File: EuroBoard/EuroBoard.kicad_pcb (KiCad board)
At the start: 2 copper layers, 100 x 100 mm, 21 parts, among them J1 SPI, SW1 RESET, SW2 BOOT, U1 AMS1117-3.3, U2 STM32G030CxT, Y1 NX2520 16MHz

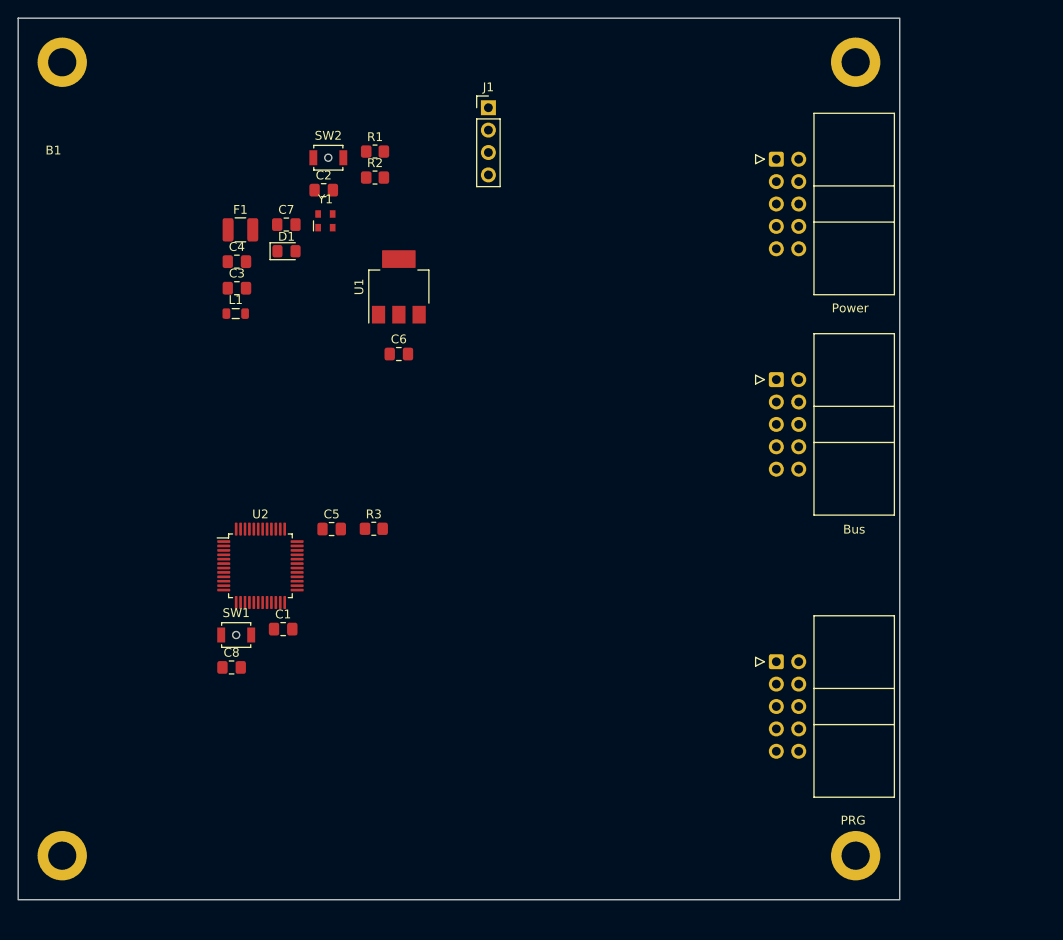
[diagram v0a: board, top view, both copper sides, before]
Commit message: Started doing PCB
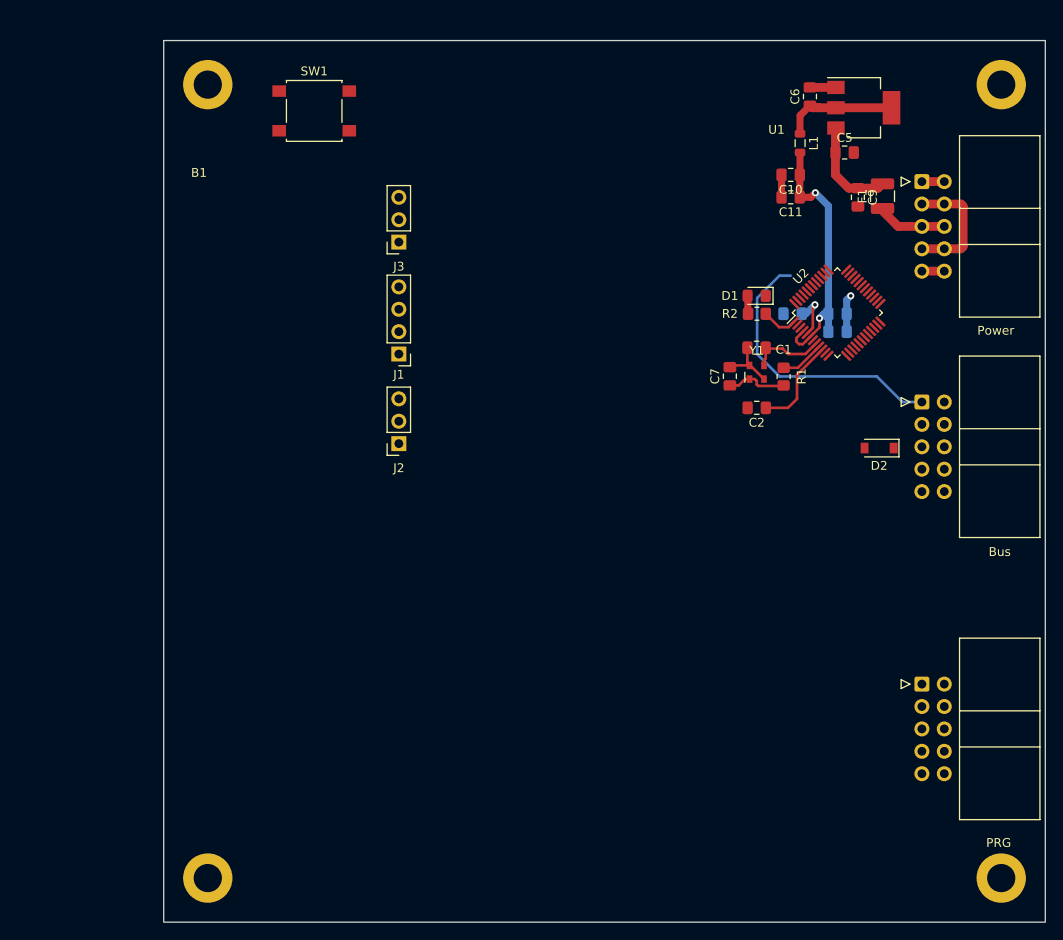
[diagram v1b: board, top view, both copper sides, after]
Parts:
- removed R3: R, Resistor_SMD:R_0805_2012Metric_Pad1.20x1.40mm_HandSolder
- removed SW2: BOOT, Button_Switch_SMD:SW_SPST_B3U-1000P-B
- added C10: 100n, Capacitor_SMD:C_0805_2012Metric_Pad1.18x1.45mm_HandSolder, F.Cu at (146.1, 48.3)
- added C11: 10u, Capacitor_SMD:C_0805_2012Metric_Pad1.18x1.45mm_HandSolder, F.Cu at (146.1, 50.8)
- added C9: 10u, Capacitor_SMD:C_0805_2012Metric_Pad1.18x1.45mm_HandSolder, F.Cu at (153.7, 50.8)
- added D2: 1n4148, Diode_SMD:D_SOD-123, F.Cu at (156.1, 79.2)
- added J2: I2C, Connector_PinSocket_2.54mm:PinSocket_1x03_P2.54mm_Vertical, F.Cu at (101.6, 78.7)
- added J3: UART, Connector_PinSocket_2.54mm:PinSocket_1x03_P2.54mm_Vertical, F.Cu at (101.6, 55.9)
- C3, C8: moved to B.Cu
- C4: value 4.7u -> 10u; moved to B.Cu
- SW1: footprint Button_Switch_SMD:SW_SPST_B3U-1000P-B -> Button_Switch_SMD:SW_SPST_B3S-1000
- moved C8 75.2 mm to (146.3, 64.0), turned to 180 degrees
- moved F1 72.9 mm to (156.5, 50.7), turned to 90 degrees
- moved C5 72.2 mm to (152.2, 45.7)
- moved U2 71.5 mm to (151.3, 63.9), turned to 45 degrees
- moved C4 68.6 mm to (151.4, 66.0)
- moved C3 68.2 mm to (151.4, 64.0)
- moved L1 66.9 mm to (147.1, 44.7), turned to -90 degrees
- moved C1 62.5 mm to (142.2, 67.9), turned to 180 degrees
- moved SW1 60.1 mm to (92.0, 41.0)
- moved U1 56.5 mm to (154.3, 40.6), turned to 0 degrees
- moved C6 55.0 mm to (148.2, 39.4), turned to 90 degrees
- moved C2 55.0 mm to (142.2, 74.7), turned to 180 degrees
- moved D1 53.6 mm to (142.2, 62.0), turned to 180 degrees
- moved C7 53.2 mm to (139.1, 71.1), turned to 90 degrees
- moved R1 52.9 mm to (145.2, 71.1), turned to 90 degrees
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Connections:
- net Net-(R2-Pad2) renamed /LED
- C2 pad 1: /RST -> Net-(C2-Pad1)
- C6 pad 1: +3.3V -> Net-(L1-Pad1)
- C8 pad 1: +3.3V -> /VREF
- F1 pad 2: Net-(F1-Pad2) -> Net-(C5-Pad1)
- L1 pad 1: Net-(F1-Pad2) -> Net-(L1-Pad1)
- L1 pad 2: Net-(C5-Pad1) -> +3.3V
- SW1 pad 2: /RST -> Net-(C2-Pad1)
- U1 pad 2: +3.3V -> Net-(L1-Pad1)
- U2 pad 10: /RST -> Net-(C2-Pad1)
- U2 pad 29: /SCL -> /TX_AUX
- U2 pad 32: /SDA -> /RX_AUX
- U2 pad 45: unconnected-(U2-Pad45) -> /SCL
- U2 pad 46: unconnected-(U2-Pad46) -> /SDA
- U2 pad 5: +3.3V -> /VREF
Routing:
- net /SCL: track 0.00 -> 32.2 mm
- net +3.3V: track 0.00 -> 30.8 mm, vias 0 -> 2
- net GND: track 0.00 -> 30.6 mm, vias 0 -> 1
- net Net-(L1-Pad1): track 0.00 -> 13.4 mm
- net Net-(C5-Pad1): track 0.00 -> 11.5 mm
- net Net-(C2-Pad1): track 0.00 -> 10.7 mm
- net /OSC_IN: track 0.00 -> 8.60 mm
- net +5V: track 0.00 -> 7.74 mm
- net Net-(C7-Pad1): track 0.00 -> 6.98 mm
- net /VREF: track 0.00 -> 5.62 mm, vias 0 -> 1
- net /OSC_OUT: track 0.00 -> 5.04 mm
- net /LED: track 0.00 -> 4.14 mm
- net -12V: track 0.00 -> 2.54 mm
- net +12V: track 0.00 -> 2.54 mm
- net Net-(D1-Pad2): track 0.00 -> 2.05 mm
